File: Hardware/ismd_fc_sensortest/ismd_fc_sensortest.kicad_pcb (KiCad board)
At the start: 2 copper layers, 28 parts, among them U1 TEENSY_4.1

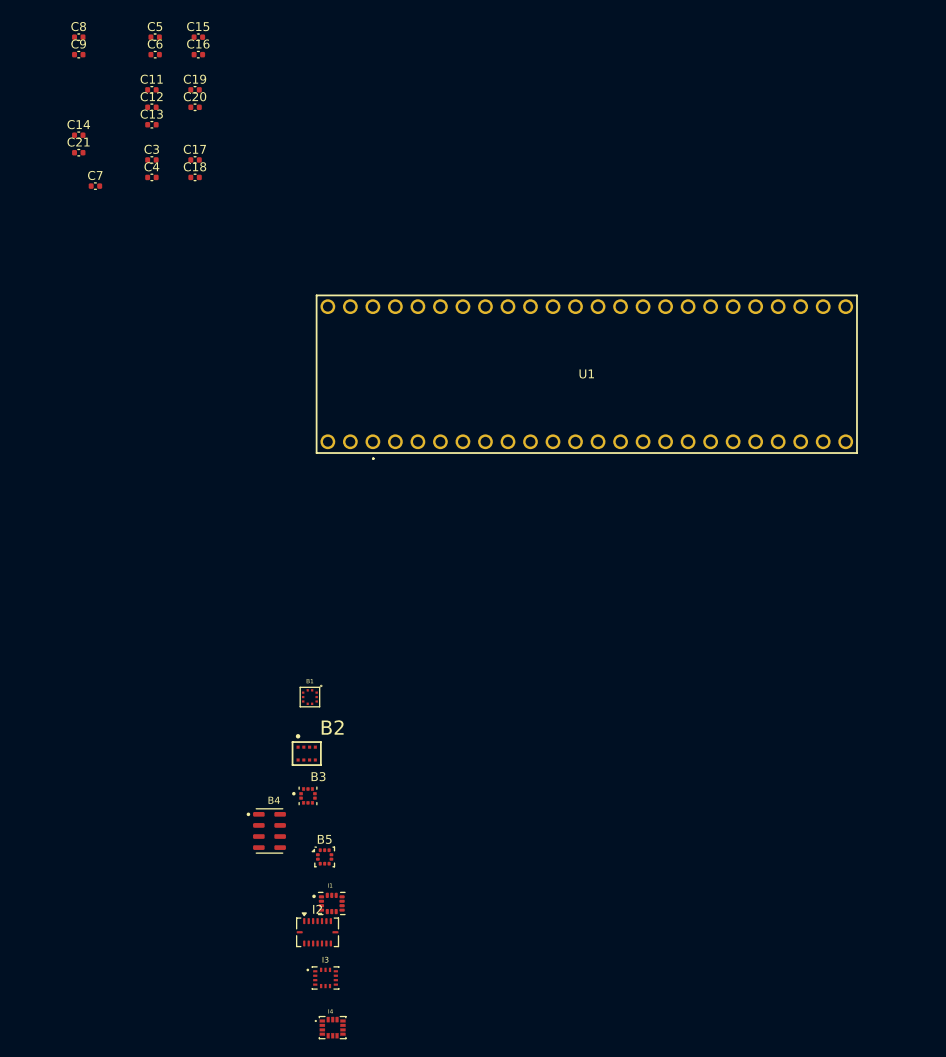
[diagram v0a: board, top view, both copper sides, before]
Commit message: sensortest work
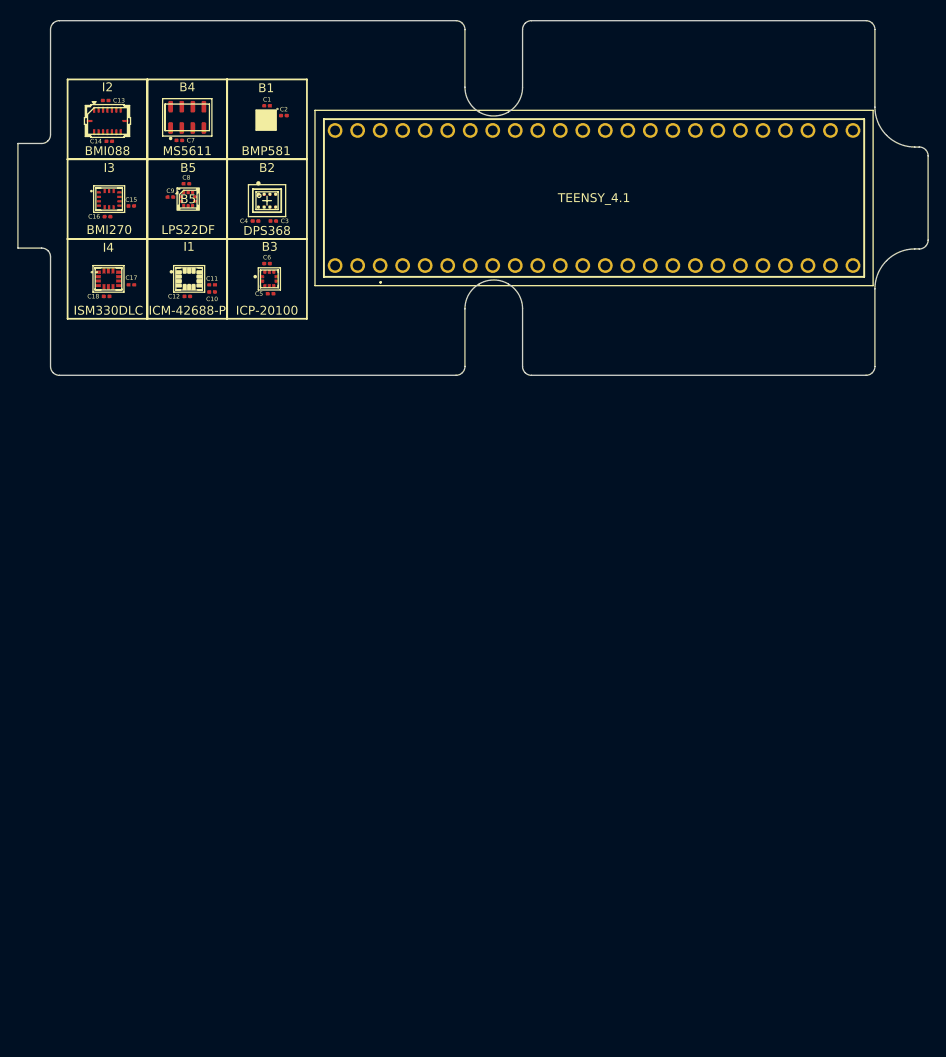
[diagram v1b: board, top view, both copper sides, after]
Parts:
- removed C19, C20, C21: 100nF, Capacitor_SMD:C_0402_1005Metric
- added C1: 100nF, Capacitor_SMD:C_0201_0603Metric, F.Cu at (42.5, 25.0)
- added C10: 0.1uF, Capacitor_SMD:C_0201_0603Metric, F.Cu at (36.3, 46.0)
- added C2: 100nF, Capacitor_SMD:C_0201_0603Metric, F.Cu at (44.4, 26.1)
- C11: value 0.1uF -> 2.2uF; footprint Capacitor_SMD:C_0402_1005Metric -> Capacitor_SMD:C_0201_0603Metric
- C12: value 2.2uF -> 10nF; footprint Capacitor_SMD:C_0402_1005Metric -> Capacitor_SMD:C_0201_0603Metric
- C13: value 10nF -> 100nF; footprint Capacitor_SMD:C_0402_1005Metric -> Capacitor_SMD:C_0201_0603Metric
- C14, C15, C16, C17, C18, C3, C4, C5, C6, C7, C8, C9: footprint Capacitor_SMD:C_0402_1005Metric -> Capacitor_SMD:C_0201_0603Metric
- I4: value ISM330DLCTR -> ISM330DLC
- moved I2 94.5 mm to (24.5, 26.7)
- moved I3 91.2 mm to (24.7, 35.5)
- moved I4 88.2 mm to (24.6, 44.5)
- moved B4 81.0 mm to (33.5, 26.3), turned to 90 degrees
- moved B5 75.8 mm to (33.6, 35.5)
- moved I1 72.3 mm to (33.7, 44.5)
- moved B1 65.3 mm to (42.4, 26.6)
- moved B2 62.5 mm to (42.5, 35.7)
- moved B3 58.5 mm to (42.8, 44.5)
- moved C5 31.7 mm to (42.9, 46.2)
- moved C6 26.7 mm to (42.5, 42.8), turned to 180 degrees
- moved C11 23.0 mm to (36.3, 45.2), turned to 180 degrees
- moved C12 21.7 mm to (33.5, 46.5)
- moved C16 20.9 mm to (24.5, 37.5)
- moved C8 20.5 mm to (33.4, 33.8), turned to 180 degrees
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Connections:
- C12 pad 1: GND -> +3V3
- C12 pad 2: +3V3 -> GND
- C16 pad 1: GND -> +3V3
- C16 pad 2: +3V3 -> GND
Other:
- board outline added: 102.7 x 40 mm
